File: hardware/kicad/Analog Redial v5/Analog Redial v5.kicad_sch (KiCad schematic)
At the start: 75 parts, among them J1 Barrel_Jack_PTH_Slot, J2 PINHD_1x8_Male, J3 PINHD_1x2_Male, J4 PINHD_1x2_Male, J5 PINHD_2x4_Male, J7 PINHD_1x3_Male, J8 RJ12, J9 RJ12, U1 ESP32-C6-DevKitC-1, U2 ES8388, U3 AG1171, U4 AG1171, U5 XC6206P332MR

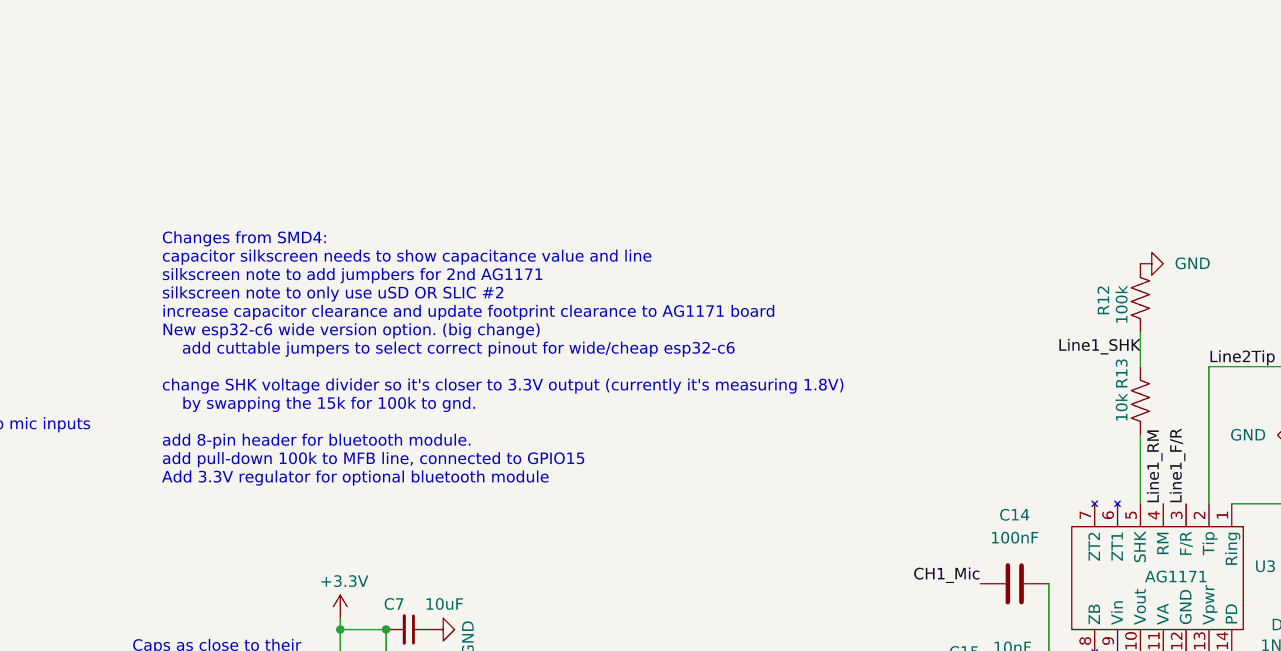
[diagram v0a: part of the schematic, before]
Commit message: KiCad v5: edits as of 2026-10-19
Co-Authored-By: Claude Opus 5.5 <noreply@anthropic.com>
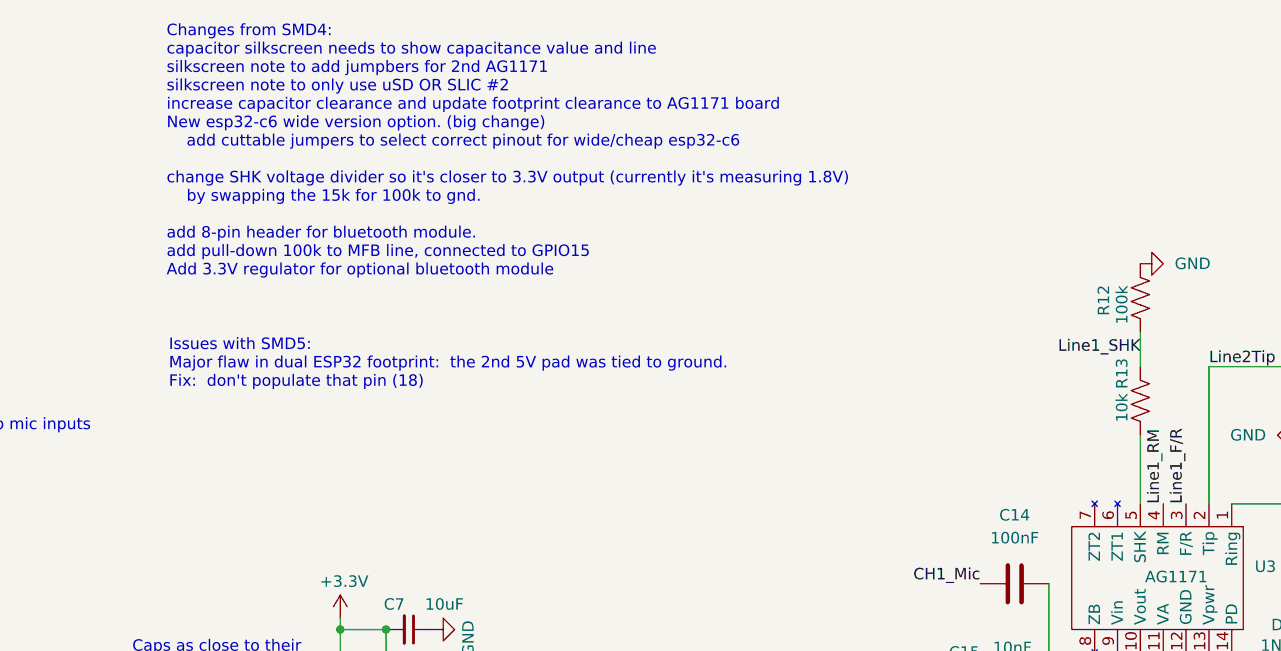
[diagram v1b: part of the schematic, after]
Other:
- note added: "Issues with SMD5: Major flaw in dual ESP32 footprint: the 2nd 5V pad was tied to ground. Fix: don't populate that pin (18)"
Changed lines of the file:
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@@
+		)
+	)
+	(text "Issues with SMD5:\nMajor flaw in dual ESP32 footprint:  the 2nd 5V pad was tied to ground. \nFix:  don't populate that pin (18)"
+		(exclude_from_sim no)
+		(at 199.39 60.706 0)
+		(effects
+			(font
+				(size 1.27 1.27)
+			)
+			(justify left)
 		)
 	)
@@
 	(text "Changes from SMD4:\ncapacitor silkscreen needs to show capacitance value and line\nsilkscreen note to add jumpbers for 2nd AG1171\nsilkscreen note to only use uSD OR SLIC #2\nincrease capacitor clearance and update footprint clearance to AG1171 board\nNew esp32-c6 wide version option. (big change)\n	add cuttable jumpers to select correct pinout for wide/cheap esp32-c6\n\nchange SHK voltage divider so it's closer to 3.3V output (currently it's measuring 1.8V)\n	by swapping the 15k for 100k to gnd.\n\nadd 8-pin header for bluetooth module.\nadd pull-down 100k to MFB line, connected to GPIO15\nAdd 3.3V regulator for optional bluetooth module\n\n"
 		(exclude_from_sim no)
-		(at 198.628 61.214 0)
+		(at 199.136 38.1 0)
 		(effects
 			(font
